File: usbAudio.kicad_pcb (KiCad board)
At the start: 2 copper layers, 45.2 x 15.6 mm, 35 parts, among them J1 USB_B_Micro, J2 54-00176, U1 PCM2906CDBR, U2 MAX9814, U3 TCR2EF36, Y1 12MHz

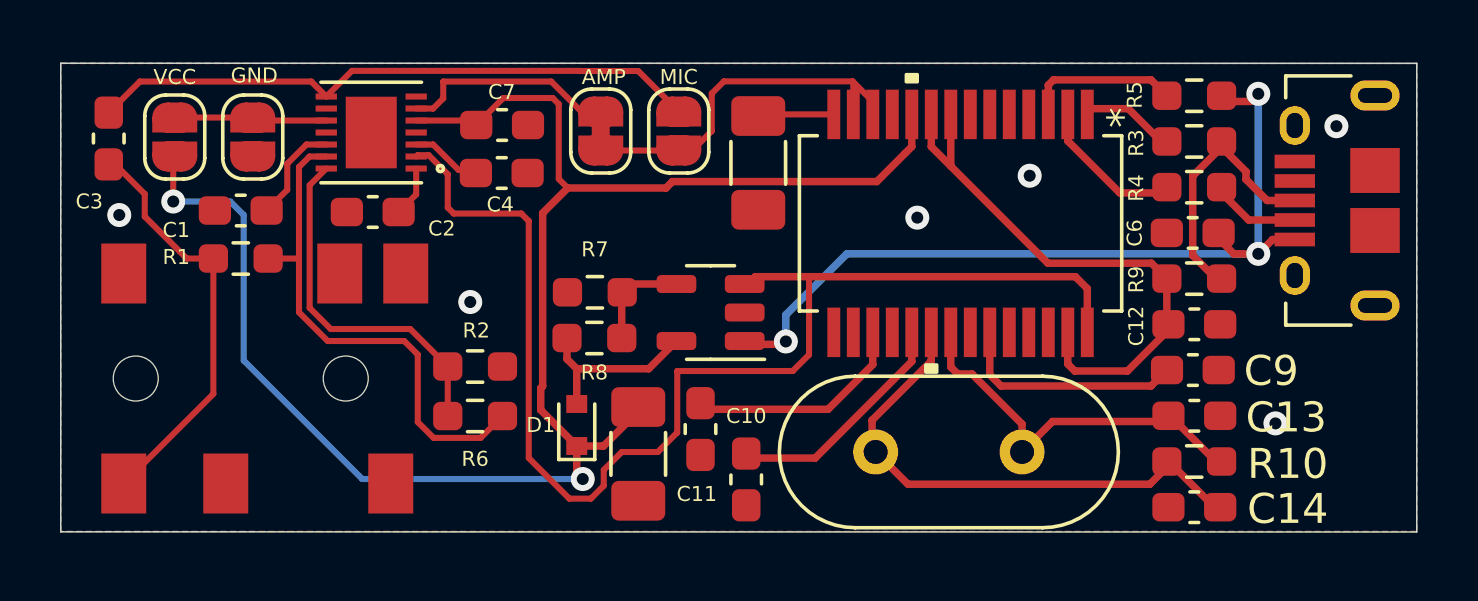
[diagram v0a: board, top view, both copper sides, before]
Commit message: Update design and readme
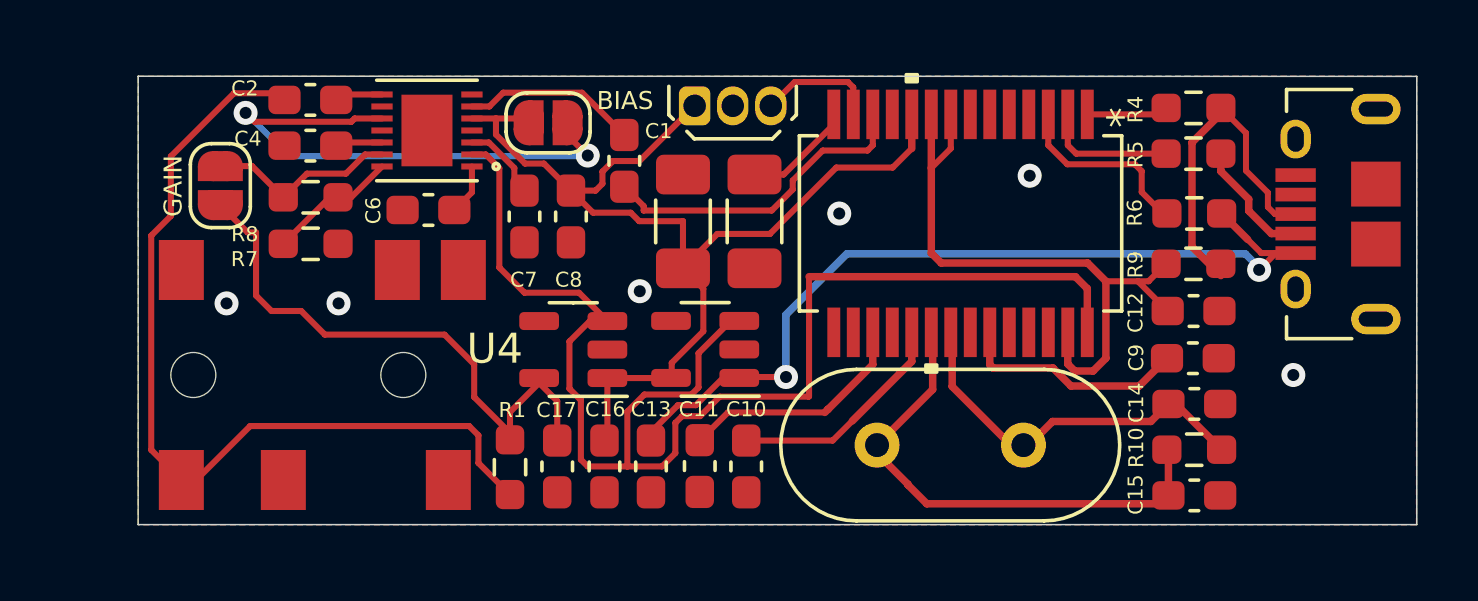
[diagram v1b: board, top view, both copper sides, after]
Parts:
- removed AMP: Jumper_NC_Small, Jumper:SolderJumper-2_P1.3mm_Bridged_RoundedPad1.0x1.5mm
- removed the C6 at (91.0, 78.3)
- removed D1: D_Schottky_Small, Diode_SMD:D_SOD-523
- removed GND, MIC: Jumper_NO_Small, Jumper:SolderJumper-2_P1.3mm_Open_RoundedPad1.0x1.5mm
- removed the R7 at (71.1, 80.3)
- removed the R8 at (71.1, 81.8)
- added C1: 0.1uF, Capacitor_SMD:C_0603_1608Metric_Pad1.08x0.95mm_HandSolder, F.Cu at (72.1, 75.9)
- added C13: 1uF, Capacitor_SMD:C_0603_1608Metric_Pad1.08x0.95mm_HandSolder, F.Cu at (73.0, 86.1)
- added C16: 1uF, Capacitor_SMD:C_0603_1608Metric_Pad1.08x0.95mm_HandSolder, F.Cu at (71.4, 86.1)
- added C17: 1uF, Capacitor_SMD:C_0603_1608Metric_Pad1.08x0.95mm_HandSolder, F.Cu at (69.8, 86.1)
- added J2: Conn_01x03, Package_TO_SOT_THT:TO-92Flat, F.Cu at (74.4, 74.1)
- added JP2: Jumper_NO_Small, Jumper:SolderJumper-2_P1.3mm_Open_RoundedPad1.0x1.5mm, F.Cu at (58.6, 76.7)
- added U4: MIC5365-3.3YD5, Package_TO_SOT_SMD:SOT-23-5, F.Cu at (70.4, 82.2)
- U3: footprint Package_TO_SOT_SMD:TSOT-23-5 -> Package_TO_SOT_SMD:SOT-23-5
- moved JP1 12.5 mm to (69.5, 74.6), turned to 180 degrees
- moved R1 11.4 mm to (68.3, 86.1), turned to -90 degrees
- moved R8 9.12 mm to (61.6, 77.1), turned to 0 degrees
- moved C3 7.89 mm to (74.0, 77.9), turned to 90 degrees
- moved C2 6.84 mm to (61.6, 73.9), turned to 180 degrees
- moved R7 6.84 mm to (61.6, 78.7)
- moved R6 3.92 mm to (91.1, 77.6)
- moved C8 3.82 mm to (70.3, 77.7), turned to -90 degrees
- moved C4 3.17 mm to (61.6, 75.4)
- moved C5 1.95 mm to (76.4, 77.9)
- moved J3 1.92 mm to (55.2, 83.0)
- moved U2 1.86 mm to (65.5, 74.9)
- moved C6 1.86 mm to (65.6, 77.5)
- moved C7 1.64 mm to (68.8, 77.7), turned to -90 degrees
- moved U3 1.24 mm to (74.8, 82.2)
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- renumbered C13 to C14, C14 to C15, C3 to C2, C8 to C3, C1 to C4, C2 to C6, C4 to C7, C7 to C8, J2 to J3, VCC to JP1, R3 to R4, R4 to R5, R5 to R6, R2 to R7, R6 to R8
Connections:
- net /MICIN renamed Net-(C2-Pad1)
- net SSPND* renamed /*SSPND
- C3 pad 1: VCCCI -> /VCCCI
- C8 pad 1: VCCCI -> /VCCCI
- J1 pad 10: GND -> (no net)
- J1 pad 11: GND -> (no net)
- J1 pad S_1: GND -> (no net)
- J1 pad S_2: GND -> (no net)
- J1 pad S_3: GND -> (no net)
- J1 pad S_4: GND -> (no net)
- JP1 pad 2: VCCCI -> /VCCCI
- R1 pad 1: Net-(R1-Pad1) -> /VBIAS
- R8 pad 1: Net-(R1-Pad1) -> Net-(JP2-Pad1)
- U1 pad 10: VCCCI -> /VCCCI
- U1 pad 12: Net-(JP1-Pad2) -> Net-(C1-Pad1)
- U1 pad 13: Net-(JP1-Pad2) -> /IN_R
- U2 pad 13: Net-(R1-Pad1) -> Net-(JP2-Pad1)
- U2 pad 5: VCCCI -> /VCCCI
- U3 pad 4: Net-(R7-Pad2) -> unconnected-(U3-Pad4)
- U3 pad 5: Net-(D1-Pad2) -> /VCCCI
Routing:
- net VCCCI: track 56.5 -> 0.00 mm, vias 2 -> 0
- net /VCCCI: track 0.00 -> 35.3 mm
- net Net-(C2-Pad1): track 20.6 -> 1.34 mm
- net /VBIAS: track 0.00 -> 18.5 mm
- net Net-(R1-Pad1): track 17.1 -> 0.00 mm
- net MIC+: track 14.0 -> 28.6 mm
- net Net-(JP1-Pad1): track 5.09 -> 18.3 mm, vias 0 -> 2
- net Net-(JP1-Pad2): track 12.6 -> 0.00 mm
- net Net-(C1-Pad1): track 0.00 -> 10.8 mm
- net Net-(R7-Pad1): track 11.9 -> 4.08 mm
- net Net-(JP2-Pad1): track 0.00 -> 6.41 mm
- net Net-(D1-Pad2): track 6.04 -> 0.00 mm
- net /IN_R: track 0.00 -> 4.05 mm
- net Net-(R7-Pad2): track 3.43 -> 0.00 mm
- net /*SSPND: track 42.0 -> 45.3 mm
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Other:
- board size 45.2 x 15.6 mm -> 42.6 x 14.9 mm
- board text added: "BIAS"
- board text added: "GAIN"
